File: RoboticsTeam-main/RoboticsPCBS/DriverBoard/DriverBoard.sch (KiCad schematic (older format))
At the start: 49 parts, among them J1 B4B-XH-A(LF)(SN), J10 B8B-XH-ALFSN, J11 B8B-XH-ALFSN, J12 B8B-XH-ALFSN, J13 B8B-XH-ALFSN, J14 B6B-XH-ALFSN, J15 B8B-XH-ALFSN, J16 USB_B_Micro, J17 Conn_01x02_Male, J18 Conn_01x02_Male, J19 B2B-XH-A(LF)(SN), J2 B4B-XH-A(LF)(SN), J20 B2B-XH-A(LF)(SN), J21 B2B-XH-A(LF)(SN), J22 Conn_01x02_Male, J23 Conn_01x02_Male, J24 B4B-XH-A(LF)(SN), J25 B4B-XH-A(LF)(SN), J26 B4B-XH-A(LF)(SN), J27 B4B-XH-A(LF)(SN), J28 B4B-XH-A(LF)(SN), J29 B4B-XH-A(LF)(SN), J3 B4B-XH-A(LF)(SN), J4 B4B-XH-A(LF)(SN), J5 B4B-XH-A(LF)(SN), J6 B4B-XH-A(LF)(SN), J7 B6B-XH-ALFSN, J8 B8B-XH-ALFSN, J9 B8B-XH-ALFSN, U1 STM32F767ZITx, U2 FT230XS, U3 MCP2562-E_SN, U4 MCP2562-E_SN, U5 MCP2562-E_SN

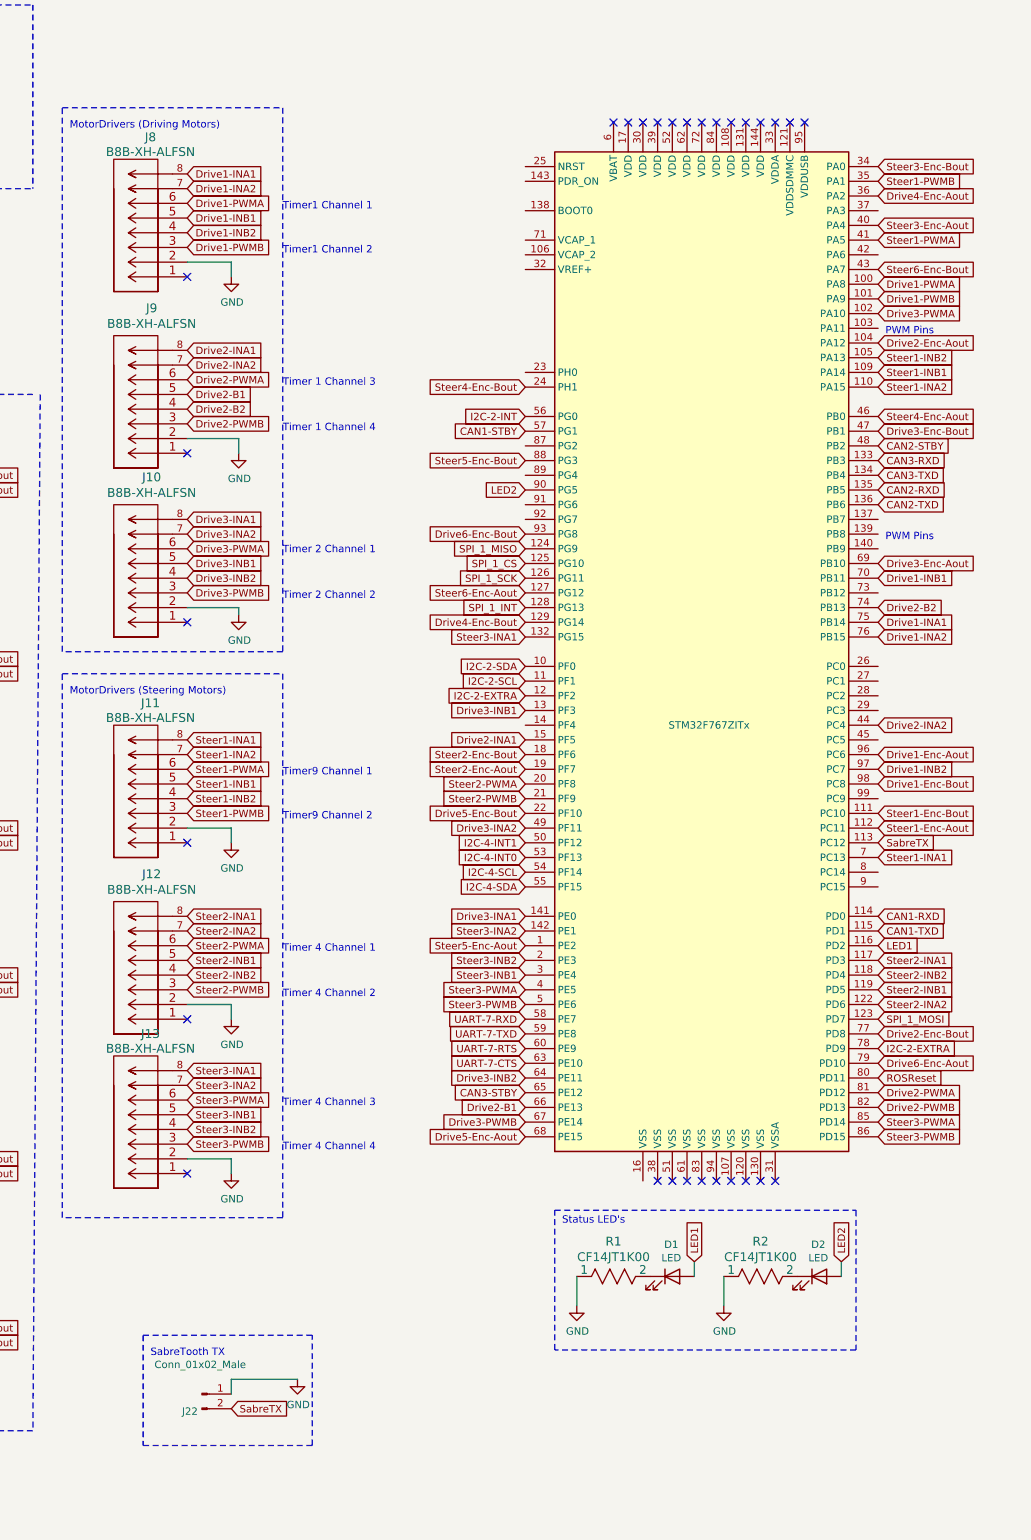
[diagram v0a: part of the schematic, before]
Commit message: Add files via upload
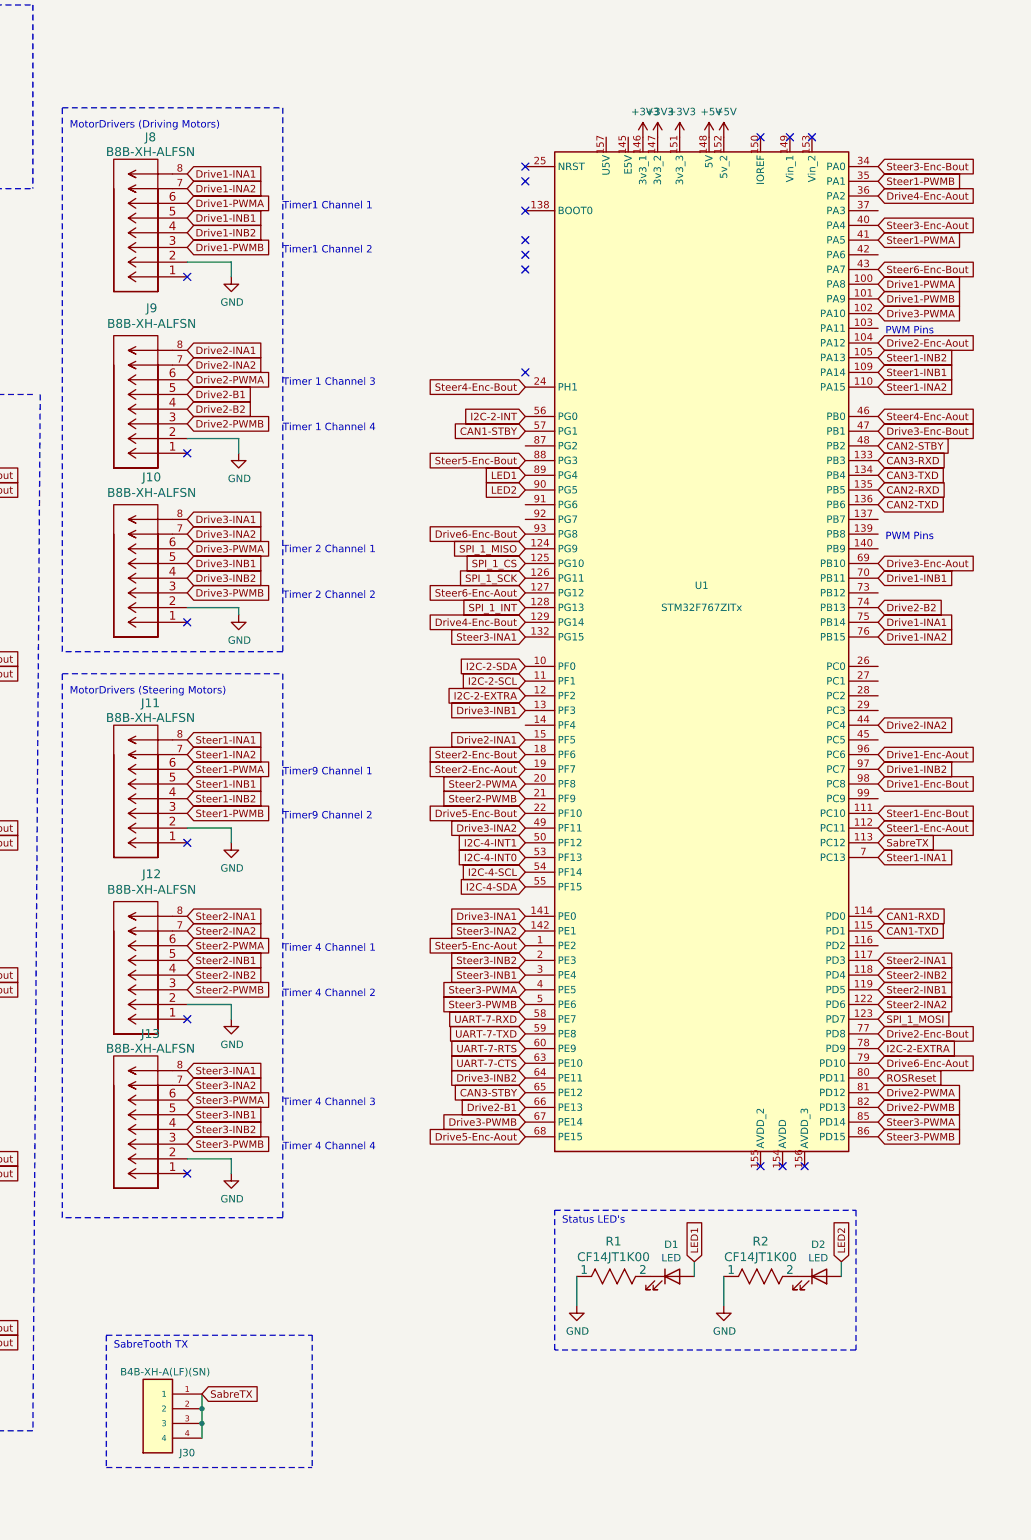
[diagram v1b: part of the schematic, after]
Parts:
- removed J22: Conn_01x02_Male, DriverBoard:2PinHeader, symbol Connector:Conn_01x02_Male
- removed U1: STM32F767ZITx, DriverBoard:STM32, symbol MCU_ST_STM32F7:STM32F767ZITx
- added J30: B4B-XH-A(LF)(SN), DriverBoard:JST4Way, symbol DriverBoard-rescue:B4B-XH-A(LF)(SN)-JST4Way
- added U1: STM32F767ZITx, DriverBoard:STM32, symbol stm32f767zitx_rev1:STM32F767ZITx
- R1, R2: footprint DriverBoard:LEDResistor -> DriverBoard:0603Footprint
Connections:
- net +3V3: now also U1.146 (3v3_1), U1.147 (3v3_2), U1.151 (3v3_3)
- net +5V: now also U1.148 (5V), U1.152 (5v_2)
- net CAN1-RXD: now also U1.114 (PD0)
- net CAN1-STBY: now also U1.57 (PG1)
- net CAN1-TXD: now also U1.115 (PD1)
- net CAN2-RXD: now also U1.135 (PB5)
- net CAN2-STBY: now also U1.48 (PB2)
- net CAN2-TXD: now also U1.136 (PB6)
- net CAN3-RXD: now also U1.133 (PB3)
- net CAN3-STBY: now also U1.65 (PE12)
- net CAN3-TXD: now also U1.134 (PB4)
- net Drive1-Enc-Aout: now also U1.96 (PC6)
- net Drive1-Enc-Bout: now also U1.98 (PC8)
- net Drive1-INA1: now also U1.75 (PB14)
- net Drive1-INA2: now also U1.76 (PB15)
- net Drive1-INB1: now also U1.70 (PB11)
- net Drive1-INB2: now also U1.97 (PC7)
- net Drive1-PWMA: now also U1.100 (PA8)
- net Drive1-PWMB: now also U1.101 (PA9)
- net Drive2-B1: now also U1.66 (PE13)
- net Drive2-B2: now also U1.74 (PB13)
- net Drive2-Enc-Aout: now also U1.104 (PA12)
- net Drive2-Enc-Bout: now also U1.77 (PD8)
- net Drive2-INA1: now also U1.15 (PF5)
- net Drive2-INA2: now also U1.44 (PC4)
- net Drive2-PWMA: now also U1.81 (PD12)
- net Drive2-PWMB: now also U1.82 (PD13)
- net Drive3-Enc-Aout: now also U1.69 (PB10)
- net Drive3-Enc-Bout: now also U1.47 (PB1)
- net Drive3-INA1: now also U1.141 (PE0)
- net Drive3-INA2: now also U1.49 (PF11)
- net Drive3-INB1: now also U1.13 (PF3)
- net Drive3-INB2: now also U1.64 (PE11)
- net Drive3-PWMA: now also U1.102 (PA10)
- net Drive3-PWMB: now also U1.67 (PE14)
- net Drive4-Enc-Aout: now also U1.36 (PA2)
- net Drive4-Enc-Bout: now also U1.129 (PG14)
- net Drive5-Enc-Aout: now also U1.68 (PE15)
- net Drive5-Enc-Bout: now also U1.22 (PF10)
- net Drive6-Enc-Aout: now also U1.79 (PD10)
- net Drive6-Enc-Bout: now also U1.93 (PG8)
- net I2C-2-EXTRA: now also U1.12 (PF2), U1.78 (PD9)
- net I2C-2-INT: now also U1.56 (PG0)
- net I2C-2-SCL: now also U1.11 (PF1)
- net I2C-2-SDA: now also U1.10 (PF0)
- net I2C-4-INT0: now also U1.53 (PF13)
- net I2C-4-INT1: now also U1.50 (PF12)
- net I2C-4-SCL: now also U1.54 (PF14)
- net I2C-4-SDA: now also U1.55 (PF15)
- net LED1: now also U1.89 (PG4)
- net LED2: now also U1.90 (PG5)
- net ROSReset: now also U1.80 (PD11)
- net SPI_1_CS: now also U1.125 (PG10)
- net SPI_1_INT: now also U1.128 (PG13)
- net SPI_1_MISO: now also U1.124 (PG9)
- net SPI_1_MOSI: now also U1.123 (PD7)
- net SPI_1_SCK: now also U1.126 (PG11)
- net SabreTX: now also J30.1, J30.2, J30.3, J30.4, U1.113 (PC12)
- net Steer1-Enc-Aout: now also U1.112 (PC11)
- net Steer1-Enc-Bout: now also U1.111 (PC10)
- net Steer1-INA1: now also U1.7 (PC13)
- net Steer1-INA2: now also U1.110 (PA15)
- net Steer1-INB1: now also U1.109 (PA14)
- net Steer1-INB2: now also U1.105 (PA13)
- net Steer1-PWMA: now also U1.41 (PA5)
- net Steer1-PWMB: now also U1.35 (PA1)
- net Steer2-Enc-Aout: now also U1.19 (PF7)
- net Steer2-Enc-Bout: now also U1.18 (PF6)
- net Steer2-INA1: now also U1.117 (PD3)
- net Steer2-INA2: now also U1.122 (PD6)
- net Steer2-INB1: now also U1.119 (PD5)
- net Steer2-INB2: now also U1.118 (PD4)
- net Steer2-PWMA: now also U1.20 (PF8)
- net Steer2-PWMB: now also U1.21 (PF9)
- net Steer3-Enc-Aout: now also U1.40 (PA4)
- net Steer3-Enc-Bout: now also U1.34 (PA0)
- net Steer3-INA1: now also U1.132 (PG15)
- net Steer3-INA2: now also U1.142 (PE1)
- net Steer3-INB1: now also U1.3 (PE4)
- net Steer3-INB2: now also U1.2 (PE3)
- net Steer3-PWMA: now also U1.4 (PE5), U1.85 (PD14)
- net Steer3-PWMB: now also U1.5 (PE6), U1.86 (PD15)
- net Steer4-Enc-Aout: now also U1.46 (PB0)
- net Steer4-Enc-Bout: now also U1.24 (PH1)
- net Steer5-Enc-Aout: now also U1.1 (PE2)
- net Steer5-Enc-Bout: now also U1.88 (PG3)
- net Steer6-Enc-Aout: now also U1.127 (PG12)
- net Steer6-Enc-Bout: now also U1.43 (PA7)
- net UART-7-CTS: now also U1.63 (PE10)
- net UART-7-RTS: now also U1.60 (PE9)
- net UART-7-RXD: now also U1.58 (PE7)
- net UART-7-TXD: now also U1.59 (PE8)
- no-connect marks 36 -> 26
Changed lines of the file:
@@
 F 0 "R1" H 8550 9488 60  0000 C CNN
 F 1 "CF14JT1K00" H 8550 9382 60  0000 C CNN
-F 2 "DriverBoard:LEDResistor" H 8550 8915 60  0001 C CNN
+F 2 "DriverBoard:0603Footprint" H 8550 8915 60  0001 C CNN
 F 3 "" H 8300 9250 60  0000 C CNN
 	1    8300 9250
@@
 F 0 "R2" H 9550 9488 60  0000 C CNN
 F 1 "CF14JT1K00" H 9550 9382 60  0000 C CNN
-F 2 "DriverBoard:LEDResistor" H 9550 8915 60  0001 C CNN
+F 2 "DriverBoard:0603Footprint" H 9550 8915 60  0001 C CNN
 F 3 "" H 9300 9250 60  0000 C CNN
 	1    9300 9250
@@
 Text GLabel 9100 9150 1    50   Input ~ 0
 LED1
-Text GLabel 10350 7000 2    50   Input ~ 0
+Text GLabel 7950 3800 0    50   Input ~ 0
 LED1
 Text GLabel 7950 3900 0    50   Input ~ 0
@@
 NoConn ~ 15150 9200
 NoConn ~ 15150 9300
-Text GLabel 5950 10150 2    50   Input ~ 0
+Text GLabel 5750 10050 2    50   Input ~ 0
 SabreTX
-Wire Notes Line style solid
-	6500 10400 6500 9650
-Wire Notes Line style solid
-	6500 9650 5350 9650
-Wire Notes Line style solid
-	5350 9650 5350 10400
-Wire Notes Line style solid
-	5350 10400 6500 10400
-Text Notes 5400 9800 0    50   ~ 0
+Text Notes 5150 9750 0    50   ~ 0
 SabreTooth TX
-$Comp
-L Connector:Conn_01x02_Male J22
-U 1 1 61C803BA
-P 5750 10050
-F 0 "J22" H 5722 9932 50  0000 R CNN
-F 1 "Conn_01x02_Male" H 6050 10250 50  0000 R CNN
-F 2 "DriverBoard:2PinHeader" H 5750 10050 50  0001 C CNN
-F 3 "~" H 5750 10050 50  0001 C CNN
-	1    5750 10050
-	1    0    0    -1
-$EndComp
-$Comp
-L power:GND #PWR0147
-U 1 1 61C8244E
-P 6400 9950
-F 0 "#PWR0147" H 6400 9700 50  0001 C CNN
-F 1 "GND" H 6405 9777 50  0000 C CNN
-F 2 "" H 6400 9950 50  0001 C CNN
-F 3 "" H 6400 9950 50  0001 C CNN
-	1    6400 9950
-	1    0    0    -1
-$EndComp
-Wire Wire Line
-	6400 9950 5950 9950
-Wire Wire Line
-	5950 9950 5950 10050
 Text GLabel 7950 7300 0    50   Input ~ 0
 Steer3-PWMA
@@
 Text GLabel 10350 7700 2    50   Input ~ 0
 I2C-2-EXTRA
-NoConn ~ 9650 8600
-NoConn ~ 9550 8600
-NoConn ~ 9450 8600
-NoConn ~ 9350 8600
-NoConn ~ 9250 8600
-NoConn ~ 9150 8600
-NoConn ~ 9050 8600
-NoConn ~ 8950 8600
-NoConn ~ 8850 8600
-NoConn ~ 9850 1400
-NoConn ~ 9750 1400
-NoConn ~ 9650 1400
-NoConn ~ 9550 1400
-NoConn ~ 9450 1400
-NoConn ~ 9350 1400
-NoConn ~ 9250 1400
-NoConn ~ 9050 1400
-NoConn ~ 9150 1400
-NoConn ~ 8550 1400
-NoConn ~ 8650 1400
-NoConn ~ 8750 1400
-NoConn ~ 8850 1400
-NoConn ~ 8950 1400
 Text GLabel 10350 5800 2    50   Input ~ 0
 Drive1-INB2
@@
 Wire Notes Line style solid
 	11750 7300 16050 7300
-$Comp
-L MCU_ST_STM32F7:STM32F767ZITx U1
-U 1 1 618DD601
-P 9150 5000
-F 0 "U1" H 9150 1200 50  0001 C CNN
-F 1 "STM32F767ZITx" H 9200 4500 50  0000 C CNN
-F 2 "DriverBoard:STM32" H 8150 1600 50  0001 R CNN
-F 3 "" H 9150 5000 50  0001 C CNN
-	1    9150 5000
-	1    0    0    -1
-$EndComp
 NoConn ~ 1350 3000
 Text Notes 10400 4250 0    50   ~ 0
@@
 Text Notes 10400 2850 0    50   ~ 0
 PWM Pins\n
+$Comp
+L stm32f767zitx_rev1:STM32F767ZITx U1
+U 1 1 61DDA08C
+P 9150 5000
+F 0 "U1" H 9150 5450 50  0000 C CNN
+F 1 "STM32F767ZITx" H 9150 5300 50  0000 C CNN
+F 2 "DriverBoard:STM32" H 8150 1600 50  0001 R CNN
+F 3 "" H 9150 5000 50  0001 C CNN
+	1    9150 5000
+	1    0    0    -1
+$EndComp
+NoConn ~ 9850 8500
+NoConn ~ 9700 8500
+NoConn ~ 9550 8500
+NoConn ~ 9900 1500
+NoConn ~ 9750 1500
+NoConn ~ 9550 1500
+$Comp
+L power:+5V #PWR0162
+U 1 1 61E321CC
+P 9300 1500
+F 0 "#PWR0162" H 9300 1350 50  0001 C CNN
+F 1 "+5V" H 9315 1673 50  0000 C CNN
+F 2 "" H 9300 1500 50  0001 C CNN
+F 3 "" H 9300 1500 50  0001 C CNN
+	1    9300 1500
+	1    0    0    -1
+$EndComp
+$Comp
+L power:+5V #PWR0163
+U 1 1 61E32E23
+P 9200 1500
+F 0 "#PWR0163" H 9200 1350 50  0001 C CNN
+F 1 "+5V" H 9215 1673 50  0000 C CNN
+F 2 "" H 9200 1500 50  0001 C CNN
+F 3 "" H 9200 1500 50  0001 C CNN
+	1    9200 1500
+	1    0    0    -1
+$EndComp
+$Comp
+L power:+3V3 #PWR0164
+U 1 1 61E33DFE
+P 9000 1500
+F 0 "#PWR0164" H 9000 1350 50  0001 C CNN
+F 1 "+3V3" H 9015 1673 50  0000 C CNN
+F 2 "" H 9000 1500 50  0001 C CNN
+F 3 "" H 9000 1500 50  0001 C CNN
+	1    9000 1500
+	1    0    0    -1
+$EndComp
+$Comp
+L power:+3V3 #PWR0165
+U 1 1 61E3489B
+P 8850 1500
+F 0 "#PWR0165" H 8850 1350 50  0001 C CNN
+F 1 "+3V3" H 8865 1673 50  0000 C CNN
+F 2 "" H 8850 1500 50  0001 C CNN
+F 3 "" H 8850 1500 50  0001 C CNN
+	1    8850 1500
+	1    0    0    -1
+$EndComp
+$Comp
+L power:+3V3 #PWR0166
+U 1 1 61E34EB9
+P 8750 1500
+F 0 "#PWR0166" H 8750 1350 50  0001 C CNN
+F 1 "+3V3" H 8765 1673 50  0000 C CNN
+F 2 "" H 8750 1500 50  0001 C CNN
+F 3 "" H 8750 1500 50  0001 C CNN
+	1    8750 1500
+	1    0    0    -1
+$EndComp
+NoConn ~ 7950 2400
+NoConn ~ 7950 2300
+NoConn ~ 7950 2200
+NoConn ~ 7950 2000
+NoConn ~ 7950 1800
+NoConn ~ 7950 1700
+NoConn ~ 7950 3100
+$Comp
+L DriverBoard-rescue:B4B-XH-A(LF)(SN)-JST4Way J30
+U 1 1 61E7B5D8
+P 5450 10250
+F 0 "J30" H 5650 10050 50  0000 C CNN
+F 1 "B4B-XH-A(LF)(SN)" H 5500 10600 50  0000 C CNN
+F 2 "DriverBoard:JST4Way" H 5450 10250 50  0001 L BNN
+F 3 "" H 5450 10250 50  0001 L BNN
+F 4 "JST Sales America Inc" H 5450 10250 50  0001 L BNN "MANUFACTURER"
+F 5 "NA" H 5450 10250 50  0001 L BNN "PARTREV"
+F 6 "Manufacturer Recommendation" H 5450 10250 50  0001 L BNN "STANDARD"
+	1    5450 10250
+	1    0    0    -1
+$EndComp
+Wire Wire Line
+	5750 10050 5750 10150
+Connection ~ 5750 10150
+Wire Wire Line
+	5750 10150 5750 10250
+Connection ~ 5750 10250
+Wire Wire Line
+	5750 10250 5750 10350
+Wire Notes Line style solid
+	6500 9650 6500 10550
+Wire Notes Line style solid
+	5100 9650 6500 9650
+Wire Notes Line style solid
+	5100 9650 5100 10550
+Wire Notes Line style solid
+	5100 10550 6500 10550
 $EndSCHEMATC
